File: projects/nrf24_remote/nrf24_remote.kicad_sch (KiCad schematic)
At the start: 72 parts, among them J1 lipo, J2 charge, J3 mic, J4 UPDI/UART, SW1 BTN0, SW2 BTN1, SW3 BTN2, U1 MCP73831-2-OT, U2 MIC5365-3.3YC5, U3 MCP6L02x-xMS, U4 LD39020DTPU18R, U5 ATtiny1616-M, U6 LSF0102YZT, U7 74LVC2T45GT, U8 nRF24L01P, U9 LSM303AH, Y1 16MHz

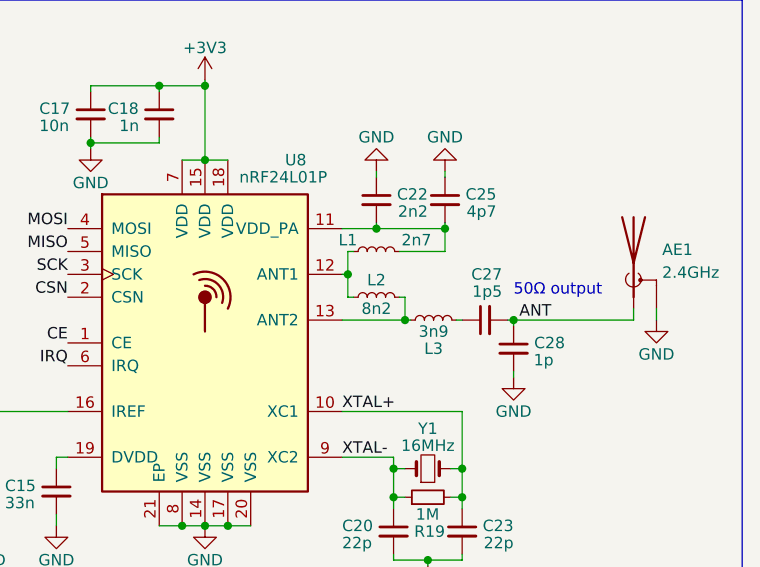
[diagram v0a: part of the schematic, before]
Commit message: move to KiCad 7
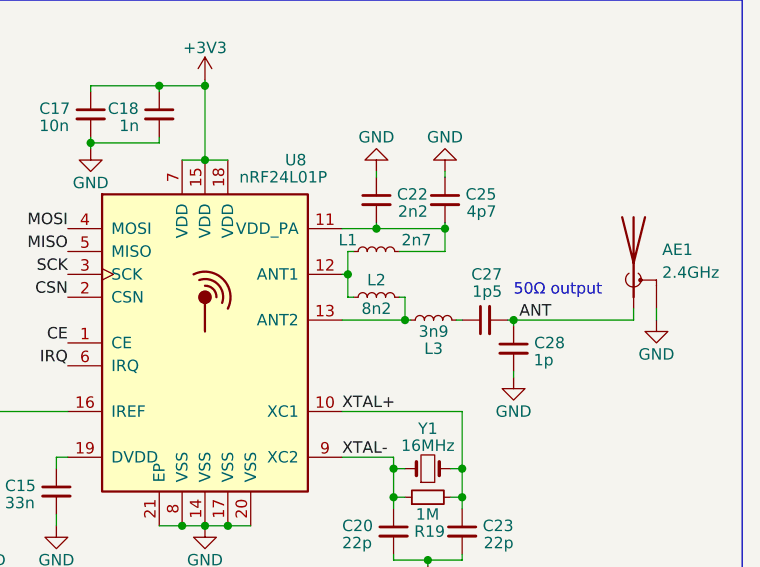
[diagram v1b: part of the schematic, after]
